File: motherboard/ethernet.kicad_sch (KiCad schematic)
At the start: 13 parts, among them U15 LPJM4938GENL, U16 TPD4EUSB30, U17 TPD4EUSB30

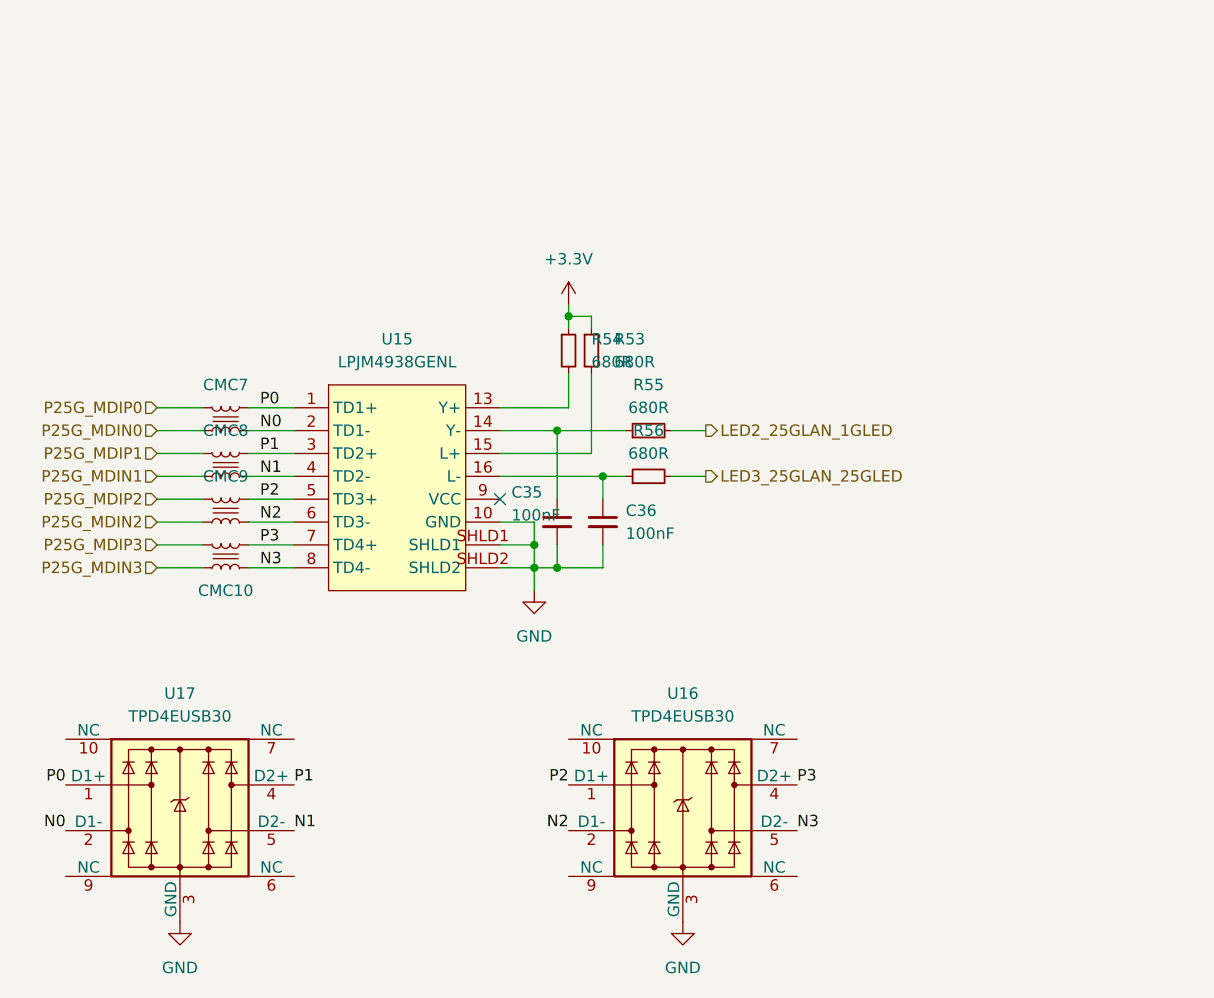
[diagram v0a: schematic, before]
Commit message: work preparing for routing
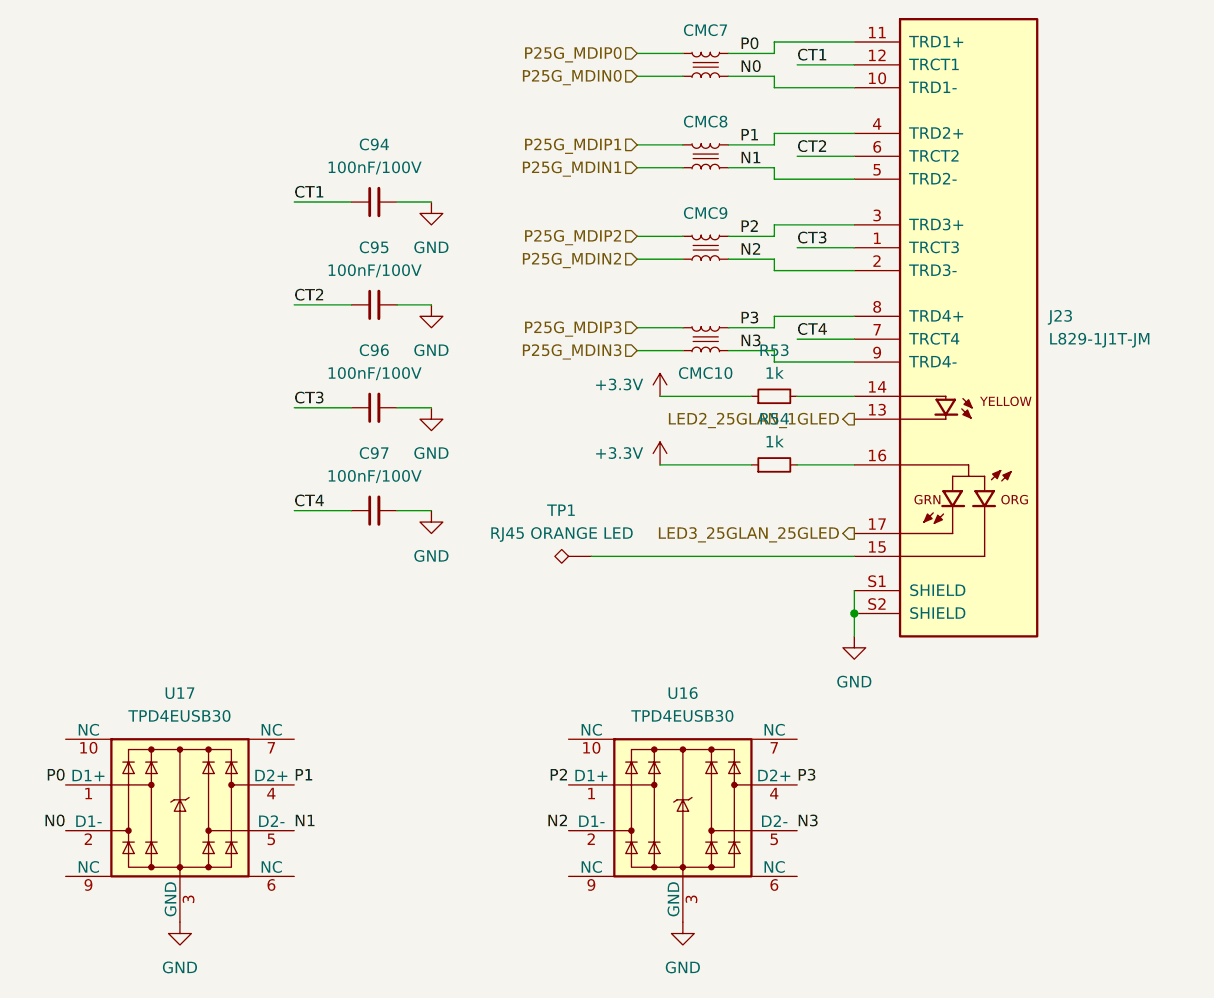
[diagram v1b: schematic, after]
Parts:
- removed C35, C36: 100nF, Capacitor_SMD:C_0402_1005Metric, symbol Device:C_Small
- removed R55, R56: 680R, Resistor_SMD:R_0402_1005Metric, symbol Device:R_Small
- removed U15: LPJM4938GENL, Connector_RJ:RJ45_Wuerth_7499111446_Horizontal, symbol library:LPJM4938GENL
- added C94, C95, C96, C97: 100nF/100V, Capacitor_SMD:C_0402_1005Metric, symbol Device:C_Small
- added J23: L829-1J1T-JM, Ethernet:BEL_L829-1J1T-JM, symbol Ethernet:L829-1J1T-JM
- added TP1: RJ45 ORANGE LED, TestPoint:TestPoint_Pad_D2.0mm, symbol Connector:TestPoint_Alt
- R53, R54: value 680R -> 1k
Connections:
- net GND: now also C94.2, C95.2, C96.2, C97.2, J23.S1 (SHIELD), J23.S2 (SHIELD)
- net LED2_25GLAN_1GLED: now also J23.13
- net LED3_25GLAN_25GLED: now also J23.17
- net N0: now also J23.10 (TRD1-)
- net N1: now also J23.5 (TRD2-)
- net N2: now also J23.2 (TRD3-)
- net N3: now also J23.9 (TRD4-)
- net P0: now also J23.11 (TRD1+)
- net P1: now also J23.4 (TRD2+)
- net P2: now also J23.3 (TRD3+)
- net P3: now also J23.8 (TRD4+)
- net at R54.2: now also J23.16
- net at R53.2: now also J23.14
- new net: J23.15, TP1.1
- new net CT1: C94.1, J23.12 (TRCT1)
- new net CT2: C95.1, J23.6 (TRCT2)
- new net CT3: C96.1, J23.1 (TRCT3)
- new net CT4: C97.1, J23.7 (TRCT4)
- no-connect marks 1 -> 0
